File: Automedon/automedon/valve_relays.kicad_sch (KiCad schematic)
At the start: 17 parts, among them J10 MS3102E14S-6S, J11 MS3102E14S-6S, J12 MS3102E14S-6S, J14 Conn_01x02_Pin, J15 Conn_01x02_Pin, J7 MS3102E14S-6S, J8 MS3102E14S-6S, J9 MS3102E14S-6S, SW2 SW_DPST_x2

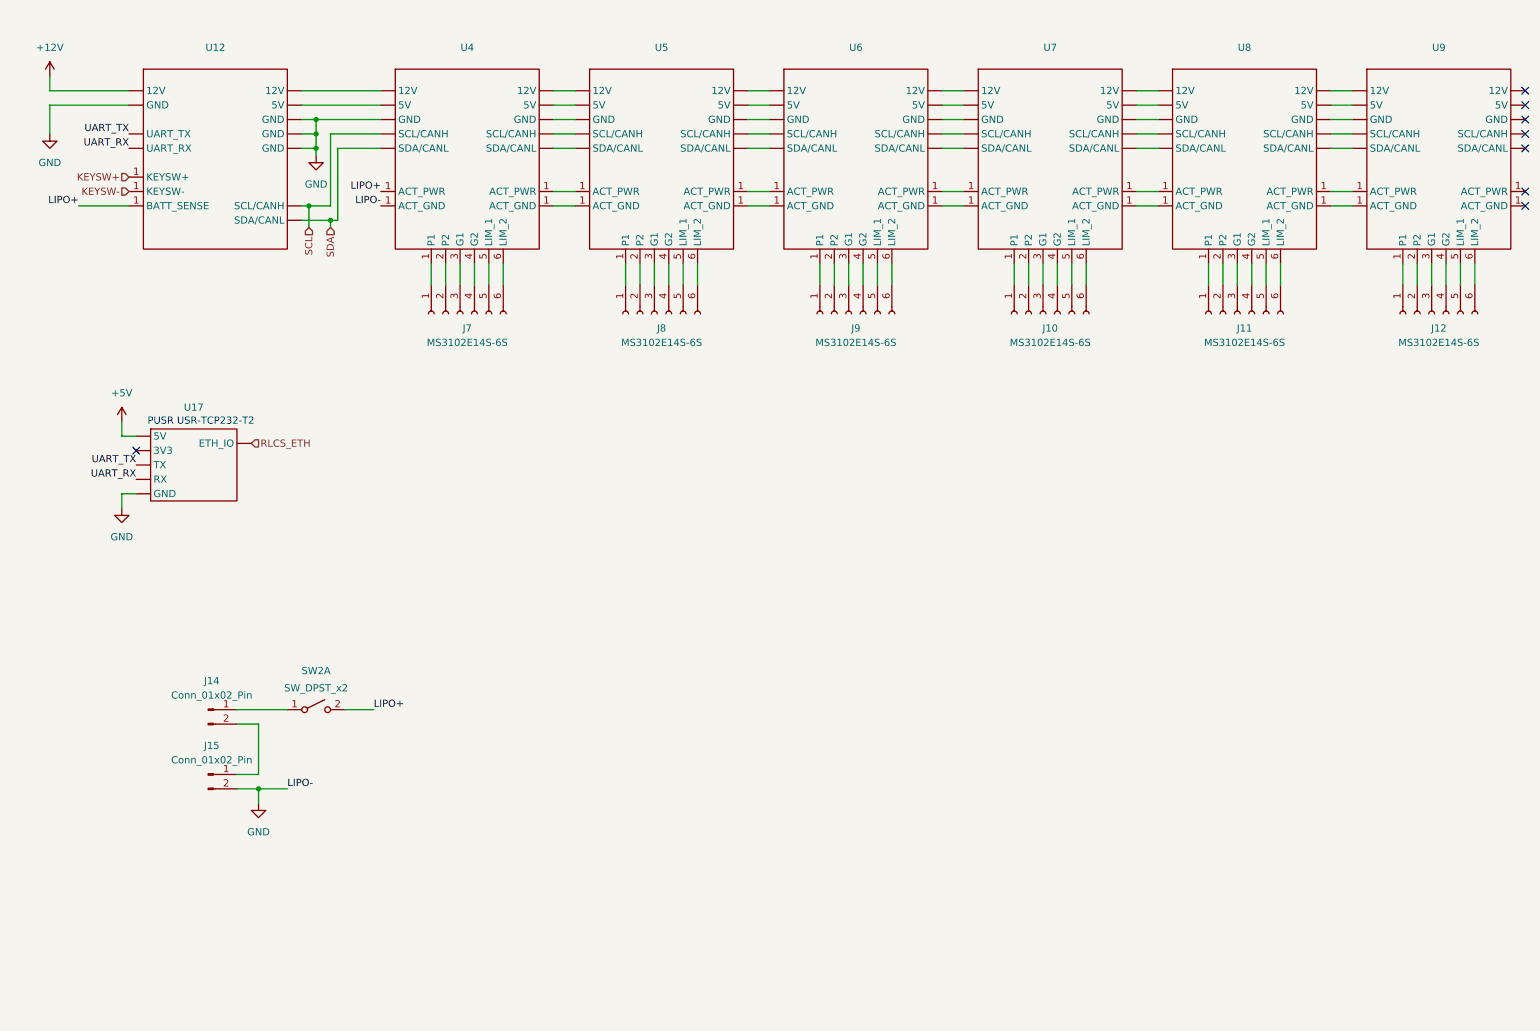
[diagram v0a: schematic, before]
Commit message: Update a bunch of shit
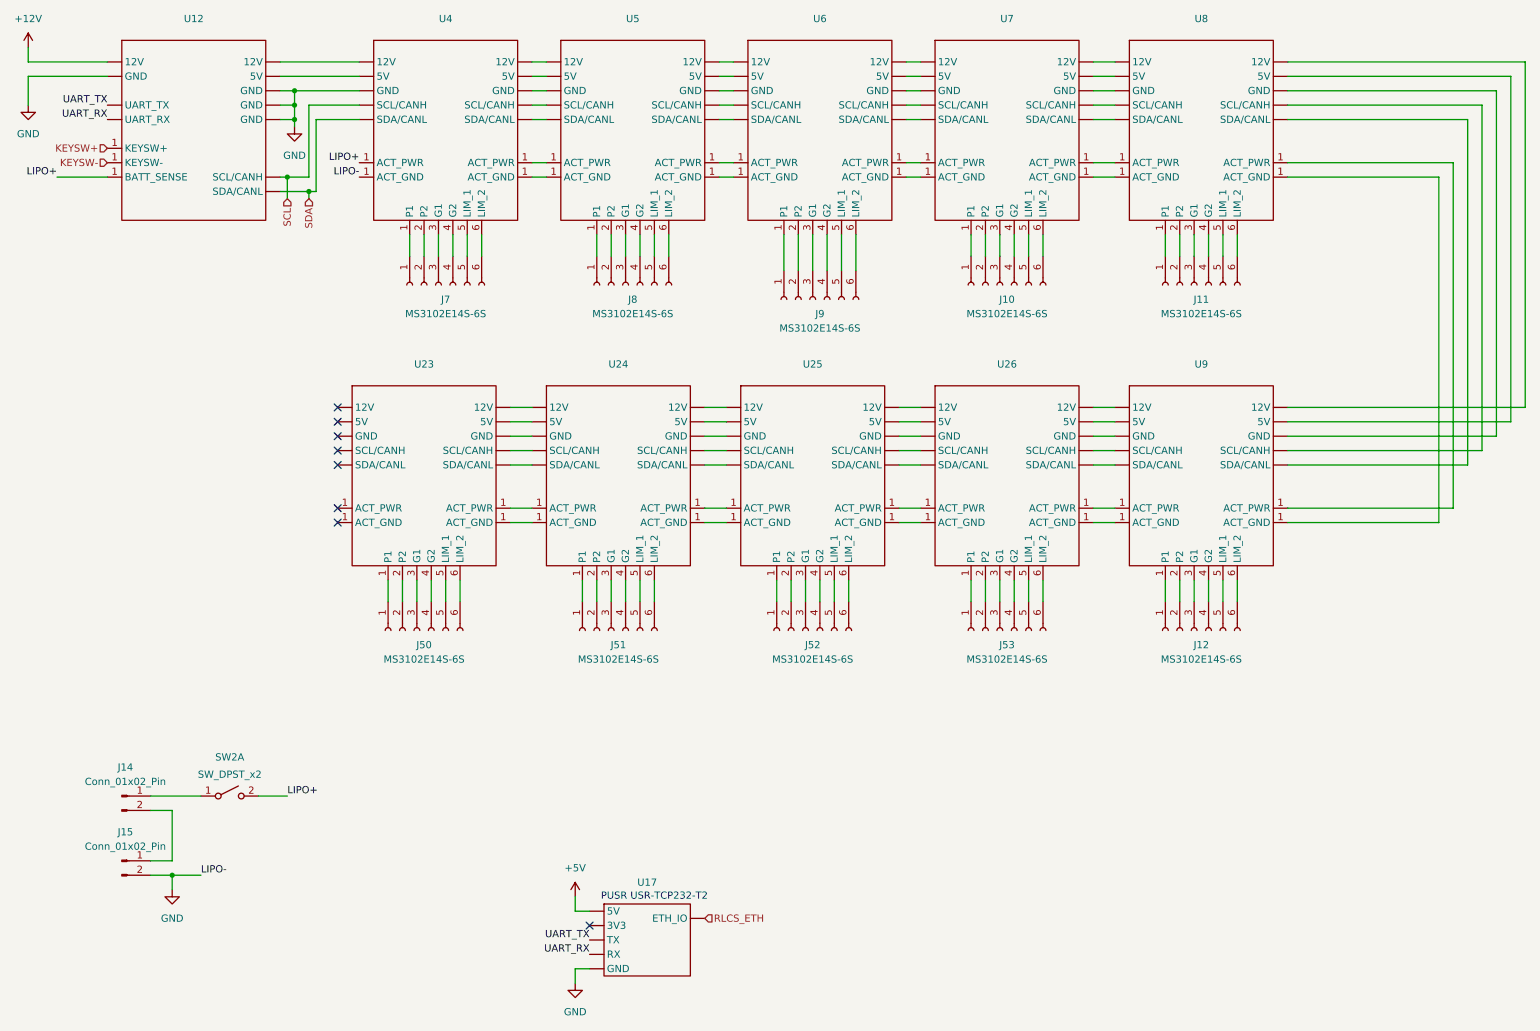
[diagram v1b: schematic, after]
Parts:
- added J50, J51, J52, J53: MS3102E14S-6S, symbol Connector:Conn_01x06_Socket
- added U23, U24, U25, U26: ~, symbol automedon:RLCS_RELAY
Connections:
- net at U5. (SDA/CANL): now also U6. (SDA/CANL); no longer U4. (SDA/CANL)
- net at U5.1 (ACT_GND): now also J8.1 (Pin_1); no longer U4.1 (ACT_GND)
- net at U6. (SDA/CANL): now also U7. (SDA/CANL); no longer U5. (SDA/CANL)
- net at U6.1 (ACT_GND): now also U7.1 (ACT_GND); no longer U5.1 (ACT_GND)
- net at U9. (SDA/CANL): now also U26. (SDA/CANL)
- net at U8. (SDA/CANL): now also U7. (SDA/CANL); no longer U9. (SDA/CANL)
- net at U9.1 (ACT_GND): now also U26.1 (ACT_GND)
- net at U8.1 (ACT_GND): now also U7.1 (ACT_GND); no longer U9.1 (ACT_GND)
- new net: U4. (SDA/CANL), U5. (SDA/CANL) (x5)
- new net: U12. (SDA/CANL), U4. (SDA/CANL) (x2)
- new net: U4.1 (ACT_GND), U5.1 (ACT_GND) (x2)
- new net: U24. (SDA/CANL), U25. (SDA/CANL) (x5)
- new net: U23. (SDA/CANL), U24. (SDA/CANL) (x5)
- new net: U24.1 (ACT_GND), U25.1 (ACT_GND) (x2)
- new net: J51.1 (Pin_1), U24.1 (ACT_GND)
- new net: U23.1 (ACT_GND), U24.1 (ACT_GND) (x2)
- new net: J51.2 (Pin_2), U24.2 (P2)
- new net: J51.3 (Pin_3), U24.3 (G1)
- new net: J51.4 (Pin_4), U24.4 (G2)
- new net: J51.5 (Pin_5), U24.5 (LIM_1)
- new net: J51.6 (Pin_6), U24.6 (LIM_2)
- new net: U5. (SDA/CANL), U6. (SDA/CANL) (x4)
- new net: U5.1 (ACT_GND), U6.1 (ACT_GND) (x2)
- new net: U25. (SDA/CANL), U26. (SDA/CANL) (x5)
- new net: J52.1 (Pin_1), U25.1 (ACT_GND)
- new net: U25.1 (ACT_GND), U26.1 (ACT_GND) (x2)
- new net: J52.2 (Pin_2), U25.2 (P2)
- new net: J52.3 (Pin_3), U25.3 (G1)
- new net: J52.4 (Pin_4), U25.4 (G2)
- new net: J52.5 (Pin_5), U25.5 (LIM_1)
- new net: J52.6 (Pin_6), U25.6 (LIM_2)
- new net: U8. (SDA/CANL), U9. (SDA/CANL) (x5)
- new net: U26. (SDA/CANL), U9. (SDA/CANL) (x4)
- new net: U8.1 (ACT_GND), U9.1 (ACT_GND) (x2)
- new net: U26.1 (ACT_GND), U9.1 (ACT_GND)
- new net: U6. (SDA/CANL), U7. (SDA/CANL) (x4)
- new net: U7. (SDA/CANL), U8. (SDA/CANL) (x4)
- new net: U6.1 (ACT_GND), U7.1 (ACT_GND)
- new net: U7.1 (ACT_GND), U8.1 (ACT_GND)
- new net: J53.1 (Pin_1), U26.1 (ACT_GND)
- new net: J53.2 (Pin_2), U26.2 (P2)
- new net: J53.3 (Pin_3), U26.3 (G1)
- new net: J53.4 (Pin_4), U26.4 (G2)
- new net: J53.5 (Pin_5), U26.5 (LIM_1)
- new net: J53.6 (Pin_6), U26.6 (LIM_2)
- new net: J50.1 (Pin_1), U23.1 (ACT_GND)
- new net: J50.2 (Pin_2), U23.2 (P2)
- new net: J50.3 (Pin_3), U23.3 (G1)
- new net: J50.4 (Pin_4), U23.4 (G2)
- new net: J50.5 (Pin_5), U23.5 (LIM_1)
- new net: J50.6 (Pin_6), U23.6 (LIM_2)
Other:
- moved on the sheet: J10, J11, J12, J14, J15, J7, J8, J9, SW2A, U12, U17, U4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
